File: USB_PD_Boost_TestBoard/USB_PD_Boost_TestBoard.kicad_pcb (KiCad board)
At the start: 2 copper layers, 83.6 x 69.8 mm, 101 parts, among them IC1 CYPD3177-24LQXQ, IC2 TPS55340PWP, J1 USB_C_Receptacle_USB2.0_16P, J3 575-4, J4 575-4, J5 575-4, J6 575-4, J7 PD_12C, Q1 SI7997DP-T1-GE3, Q2 SI7997DP-T1-GE3, Q3 IRLML0030

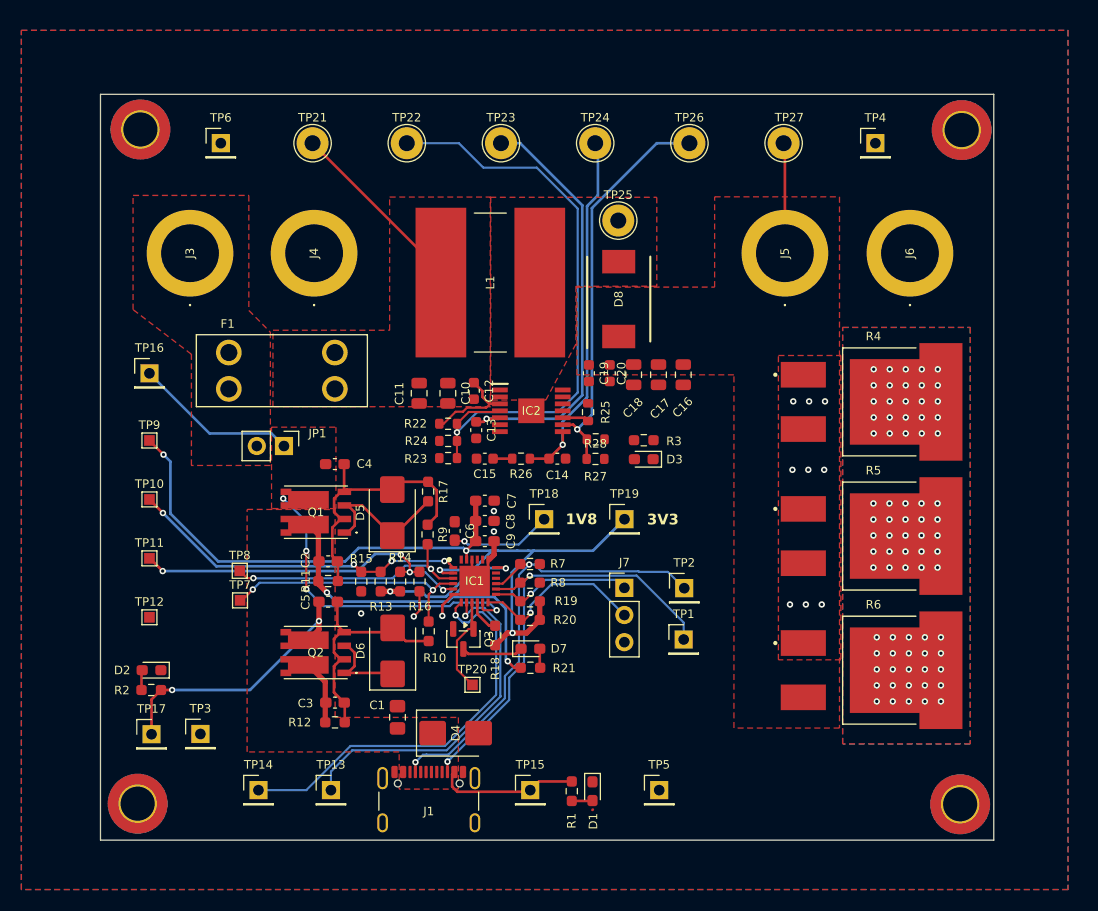
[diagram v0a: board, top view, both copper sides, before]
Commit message: cooking or no??
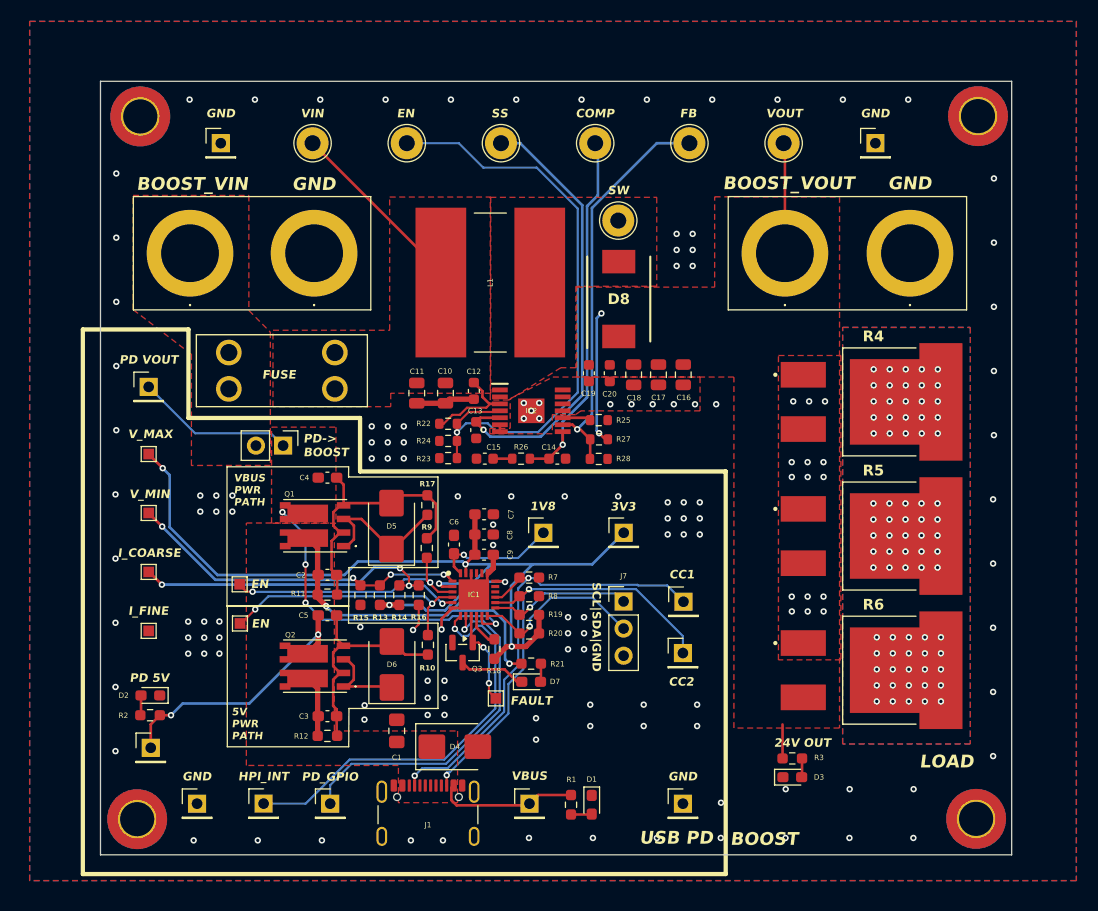
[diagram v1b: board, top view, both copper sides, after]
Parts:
- moved R3 32.9 mm to (158.6, 140.9), turned to 0 degrees
- moved D3 32.8 mm to (158.6, 142.7), turned to 0 degrees
- moved TP3 6.53 mm to (102.9, 145.2)
- moved D7 3.09 mm to (134.1, 133.8)
- moved TP5 2.56 mm to (148.3, 145.2)
- moved TP20 2.53 mm to (130.8, 135.3)
- moved D2 2.36 mm to (98.5, 135.1)
- moved R2 2.36 mm to (98.5, 136.9)
- moved TP7 2.16 mm to (106.9, 128.3)
- moved H4 2.02 mm to (175.8, 146.6)
- moved H2 2.01 mm to (175.9, 80.9)
- moved C3 1.45 mm to (115.1, 137.0)
- moved R12 1.45 mm to (115.1, 138.8)
- moved H3 1.45 mm to (97.3, 146.6)
- moved C4 1.45 mm to (115.1, 114.7)
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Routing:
- net /BOOST_24V_OUT: track 10.3 -> 26.1 mm, vias 0 -> 2
- net GND: track 14.1 -> 20.2 mm, vias 14 -> 144
- net Net-(IC2-SS): track 40.0 -> 42.3 mm
- net /USB_PD/PD_1V8: track 9.51 -> 11.6 mm
- net Net-(D3-A): track 0.00 -> 1.77 mm
- net /VBUS_IN: track 57.6 -> 56.0 mm
- net Net-(IC2-EN): track 56.3 -> 57.0 mm
- net /USB_PD/PD_HPI_INT: track 38.9 -> 38.3 mm
- net /PD_5V_OUT: track 26.0 -> 25.4 mm
- net /PD_VOUT: track 45.7 -> 45.1 mm
- net /USB_PD/PD_FAULT: track 9.28 -> 8.99 mm, vias 0 -> 2
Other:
- board size 83.6 x 69.8 mm -> 85.2 x 72.4 mm
- board text added: "24V OUT"
- board text added: "5V PWR PATH"
- board text added: "BOOST"
- board text added: "BOOST_VIN"
- board text added: "BOOST_VOUT"
- board text added: "CC1"
- board text added: "CC2"
- board text added: "COMP"
- board text added: "EN"
- board text added: "FAULT"
- board text added: "FB"
- board text added: "FUSE"
- board text added: "GND"
- board text added: "HPI_INT"
- board text added: "I_COARSE"
- board text added: "I_FINE"
- board text added: "LOAD"
- board text added: "PD 5V"
- board text added: "PD VOUT"
- board text added: "PD-> BOOST"
- board text added: "PD_GPIO"
- board text added: "SCL|SDA|GND"
- board text added: "SS"
- board text added: "SW"
- board text added: "USB PD"
- board text added: "VBUS"
- board text added: "VBUS PWR PATH"
- board text added: "VIN"
- board text added: "VOUT"
- board text added: "V_MAX"
- board text added: "V_MIN"
